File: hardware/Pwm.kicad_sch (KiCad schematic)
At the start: 69 parts, among them J10 Conn_01x03_Male, J11 Conn_01x03_Male, J12 Conn_01x03_Male, J13 Conn_01x03_Male, J14 Conn_01x03_Male, J15 Conn_01x03_Male, J16 JST XH, J17 KF350, J18 JST XH, J19 JST XH, J20 KF350, J21 JST XH, J4 JST XH, J5 KF129, J6 KF350, J7 Conn_01x03_Male, J8 Conn_01x03_Male, J9 Conn_01x03_Male, U6 74HCT04

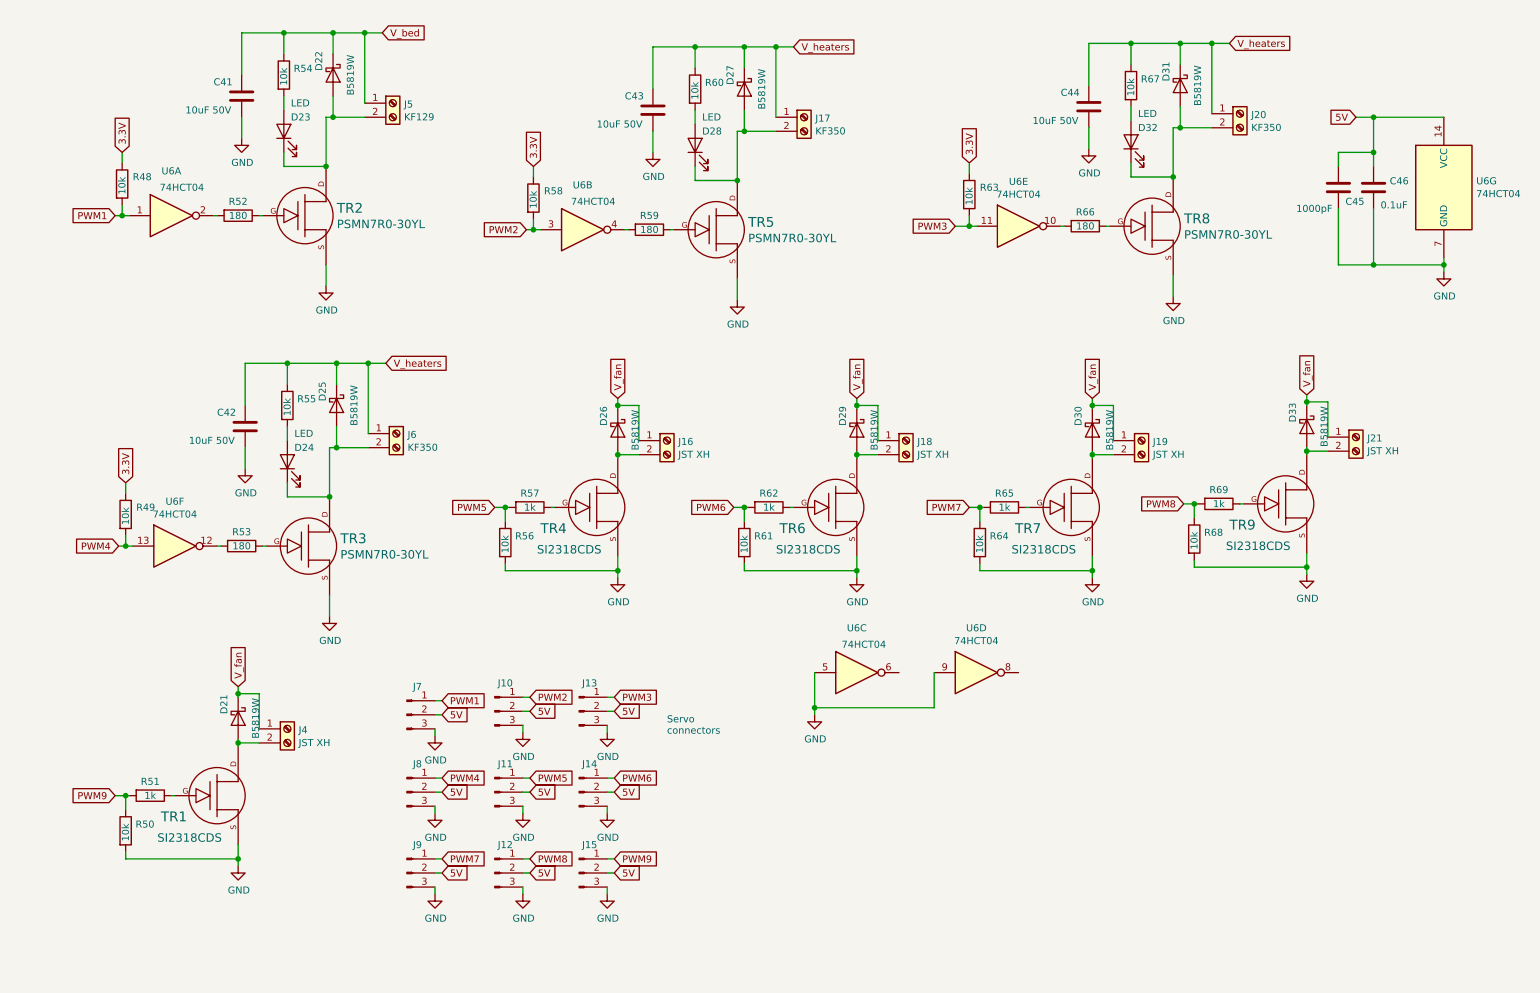
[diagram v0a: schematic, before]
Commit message: Intermediate checkin
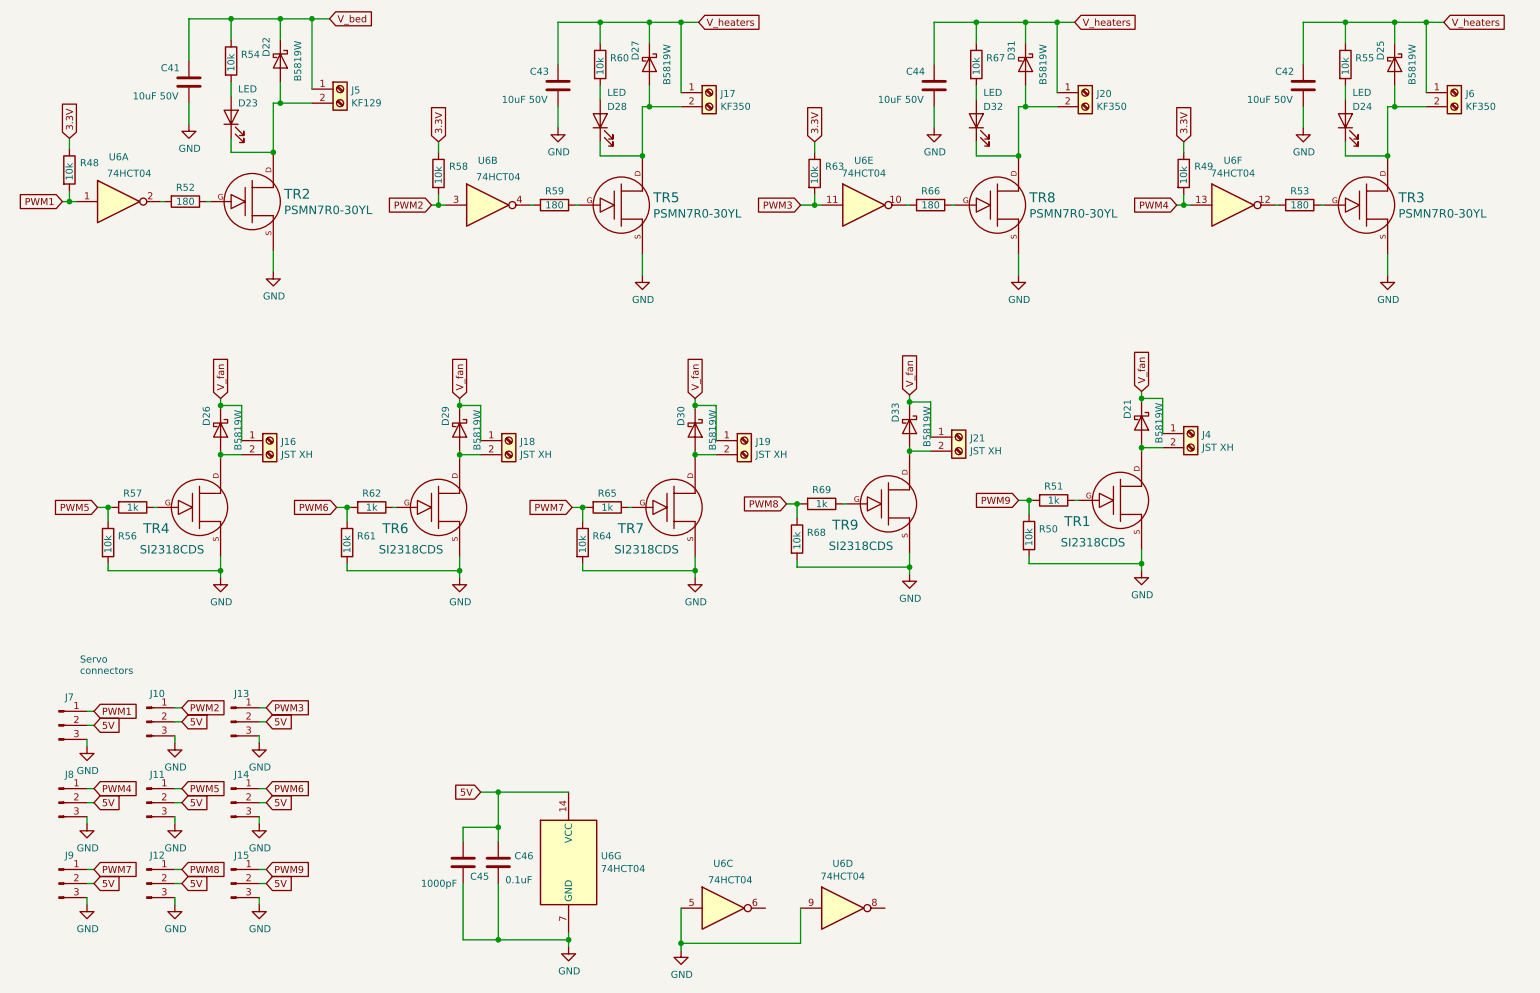
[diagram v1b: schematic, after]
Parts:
- C45: footprint PrntrBoardV2:C_0603_1608Metric -> Capacitor_SMD:C_0402_1005Metric; LCSC Part # C1588 -> C1523; Part # CL10B102KB8NNNC -> 0402B102K500NT
- C46: footprint PrntrBoardV2:C_0603_1608Metric -> Capacitor_SMD:C_0402_1005Metric; LCSC Part # C14663 -> C1525; Part # CC0603KRX7R9BB104 -> CL05B104KO5NNNC
- R48, R49, R50, R54, R55, R56, R58, R60, R61, R63, R64, R67, R68: footprint PrntrBoardV2:R_0603_1608Metric -> Resistor_SMD:R_0402_1005Metric; LCSC Part # C25804 -> C25744; Part # 0603WAF1002T5E -> 0402WGF1002TCE
- R51, R57, R62, R65, R69: footprint PrntrBoardV2:R_0603_1608Metric -> Resistor_SMD:R_0402_1005Metric; LCSC Part # C21190 -> C11702; Part # 0603WAF1001T5E -> 0402WGF1001TCE
- R52, R53, R59, R66: footprint PrntrBoardV2:R_0603_1608Metric -> Resistor_SMD:R_0603_1608Metric
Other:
- moved on the sheet: C41, C42, C43, C44, C45, C46, D21, D22, D23, D24, D25, D26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
